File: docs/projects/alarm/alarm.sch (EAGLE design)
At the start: 8 parts, among them IC2 MEGA8-P

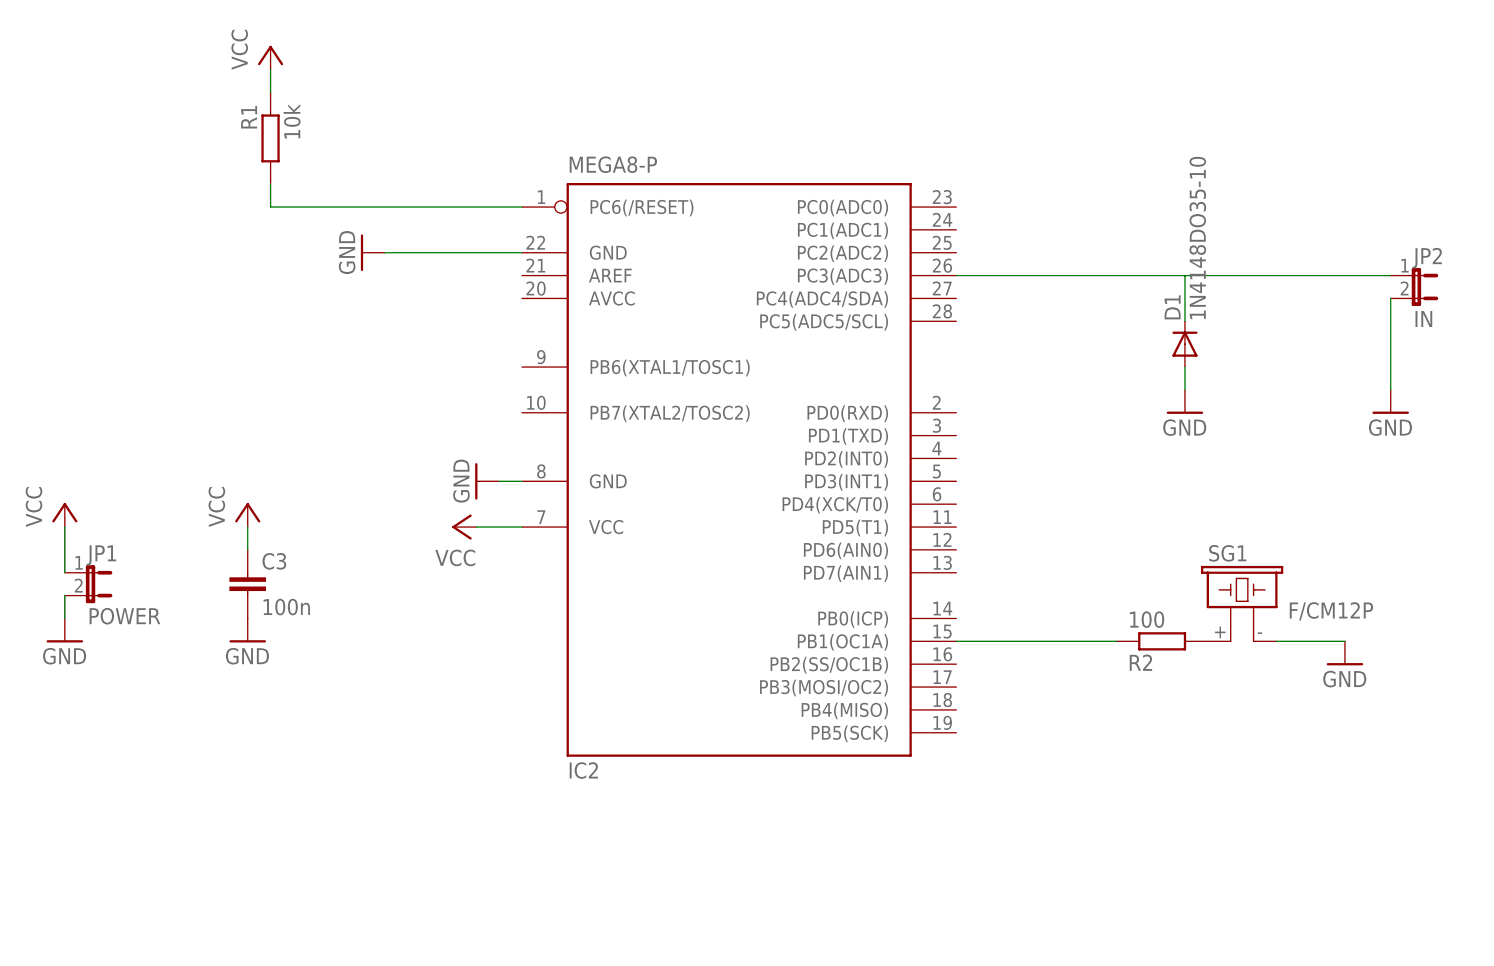
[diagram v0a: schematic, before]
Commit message: alarm: new debug
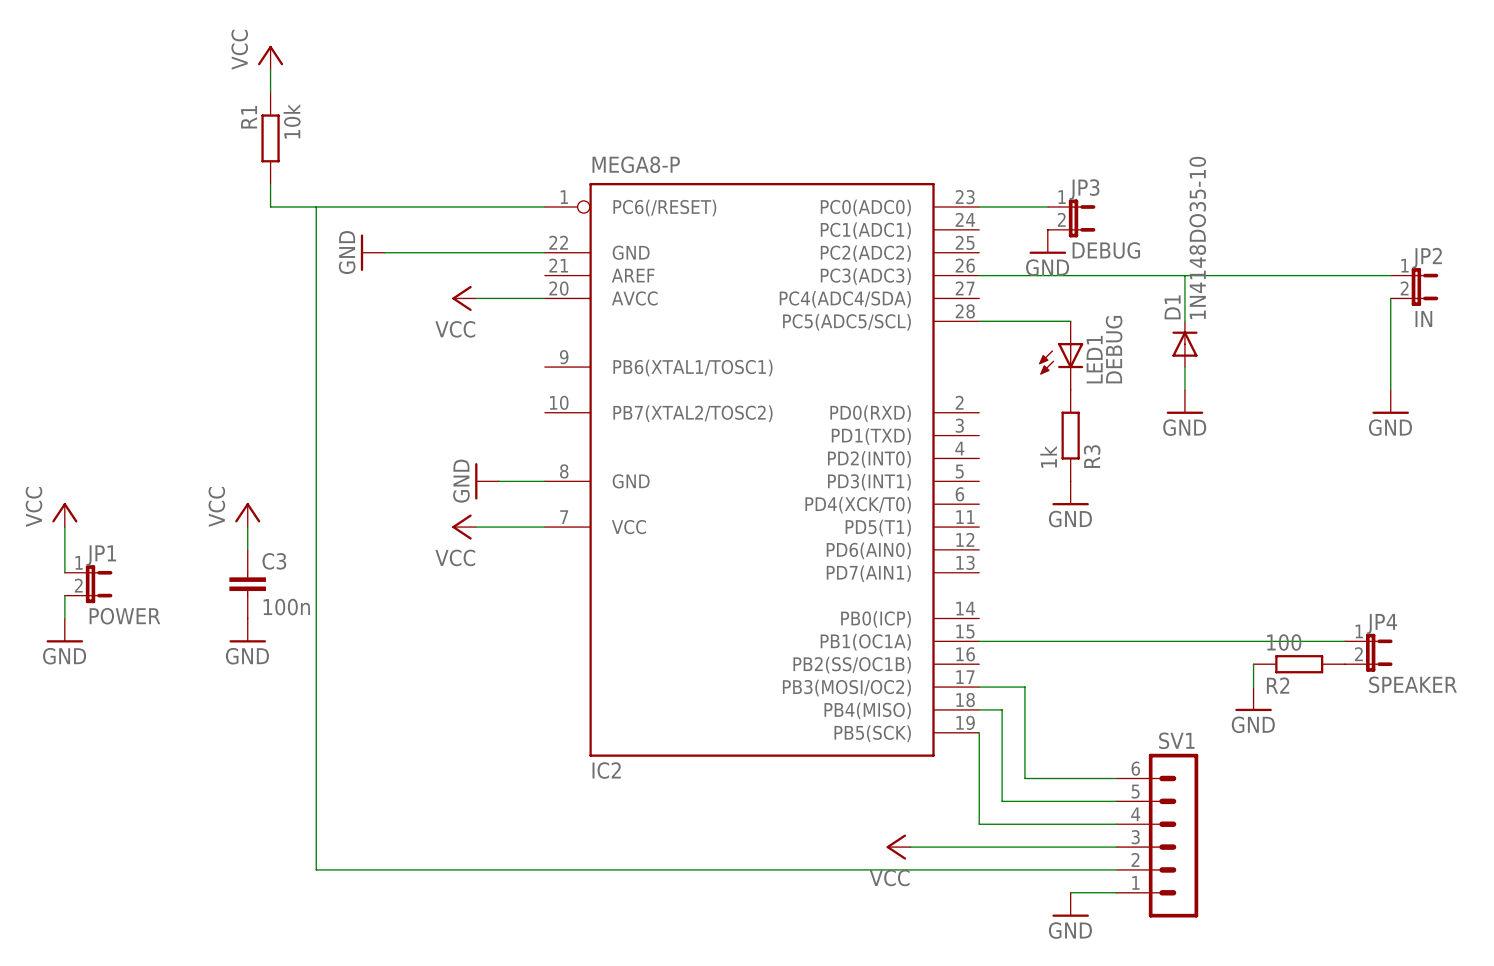
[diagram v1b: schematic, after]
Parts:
- removed SG1: F/CM12P, buzzer:F/CM12P
- added JP3: DEBUG, jumper:JP1E
- added JP4: SPEAKER, jumper:JP1E
- added LED1: DEBUG, led:LED5MM
- added R3: 1k, rcl:R-EU_0617/17
- added SV1: (no value), con-lstb:MA06-1
- R2: device rcl:R-EU_0207/10 -> rcl:R-EU_M0805
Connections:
- new net N$4: IC2.PC0(ADC0), JP3.1
- new net N$5: IC2.PB5(SCK), SV1.4
- new net N$6: IC2.PB4(MISO), SV1.5
- new net N$7: IC2.PB3(MOSI/OC2), SV1.6
- new net N$8: LED1.C, R3.2
- new net N$9: IC2.PC5(ADC5/SCL), LED1.A
- net GND: now also JP3.2, R2.1, R3.1, SV1.1; no longer SG1.2
- net N$1: now also JP4.2; no longer SG1.1
- net N$17: now also SV1.2
- net N$3: now also JP4.1; no longer R2.1
- net VCC: now also IC2.AVCC, SV1.3
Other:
- moved on the sheet: IC2, R2
